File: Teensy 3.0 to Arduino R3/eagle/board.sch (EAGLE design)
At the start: 43 parts, among them IC1 7805TV, IC2 24AA256SN, IC3 24AA256SN, IC4 24AA256SN, IC5 24AA256SN, U1 MICROSD

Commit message: Version 3 final
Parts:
- added C9: (no value), resistor:CPOL-EUD
- added D2: (no value), SparkFun-DiscreteSemi:DIODESMA-KIT
- added R10, R11, R12, R13, R14, R15, R16, R17, R18, R19, R20, R21, R22, R23, R24, R5, R6, R7, R8, R9: (no value), resistor:R-EU_R0805
- added SJ3, SJ4, SJ5, SJ6: SOLDERJUMPERNO, SparkFun-Passives:SOLDERJUMPERNO
- IC1: value 7805TV -> 78XX compatible
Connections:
- removed net 3V3: C2.+, C4.1, C5.1, C6.1, C7.1, C8.1, IC1.VO, IC2.A2, IC2.VCC, IC3.A1, IC3.A2, IC3.VCC, IC4.A0, IC4.A2, IC4.VCC, IC5.A0, IC5.A1, IC5.A2, IC5.VCC, JP12.1, JP13.13, JP14.1, JP6.5, JP6.7, R1.2, R2.2, R3.2, R4.2, SJ2.1, U1.VDD
- new net N$10: JP2.7, R10.2
- new net N$11: JP2.6, R11.2
- new net N$12: JP2.5, R12.2
- new net N$13: JP1.13, R13.2
- new net N$14: JP1.12, R14.2
- new net N$15: JP1.11, R15.2
- new net N$16: JP1.10, R16.2
- new net N$17: JP1.9, R17.2
- new net N$18: JP1.8, R18.2
- new net N$19: JP1.7, R19.2
- new net N$20: JP1.6, R20.2
- new net N$21: JP2.4, R21.2
- new net N$22: JP2.3, R22.2
- new net N$23: JP2.2, R23.2
- new net N$24: JP2.1, R24.2
- new net N$5: JP1.5, R5.2
- new net N$6: JP1.4, R6.2
- new net N$7: JP1.3, R7.2
- new net N$8: JP1.2, R8.2
- new net N$9: JP1.1, R9.2
- new net NIC: R4.1, SJ3.1, SJ4.1, U1.CARD_DETECT
- new net QW: SJ5.1, SJ6.1, U1.CS
- net 3.3V: now also C2.+, C4.1, C5.1, C6.1, C7.1, C8.1, C9.+, D2.A, IC1.VO, IC2.A2, IC2.VCC, IC3.A1, IC3.A2, IC3.VCC, IC4.A0, IC4.A2, IC4.VCC, IC5.A0, IC5.A1, IC5.A2, IC5.VCC, JP12.1, JP13.13, JP14.1, JP6.5, JP6.7, R1.2, R2.2, R3.2, R4.2, SJ2.1, U1.VDD
- net A0: now also R23.1; no longer JP2.2
- net A1: now also R22.1; no longer JP2.3
- net A2: now also R21.1; no longer JP2.4
- net A3: now also R12.1; no longer JP2.5
- net A4: now also R11.1; no longer JP2.6
- net A5: now also R10.1; no longer JP2.7
- net D0: now also R13.1; no longer JP1.13
- net D1: now also R14.1; no longer JP1.12
- net D10: now also R7.1, SJ6.2; no longer JP1.3, U1.CS
- net D11: now also R8.1; no longer JP1.2
- net D12: now also R9.1; no longer JP1.1
- net D13: now also R24.1; no longer JP2.1
- net D2: now also R15.1; no longer JP1.11
- net D3: now also R16.1; no longer JP1.10
- net D4: now also R17.1; no longer JP1.9
- net D5: now also R18.1; no longer JP1.8
- net D6: now also R19.1; no longer JP1.7
- net D7: now also R20.1, SJ3.2; no longer JP1.6
- net D8: now also R5.1, SJ4.2; no longer JP1.5, R4.1, U1.CARD_DETECT
- net D9: now also R6.1, SJ5.2; no longer JP1.4
- net GND: now also C9.-
- net N$3: now also D2.C
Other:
- moved on the sheet: BAT1, C3, C4, F2, JP1, JP11, JP12, JP13, JP14, JP15, JP2, JP3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

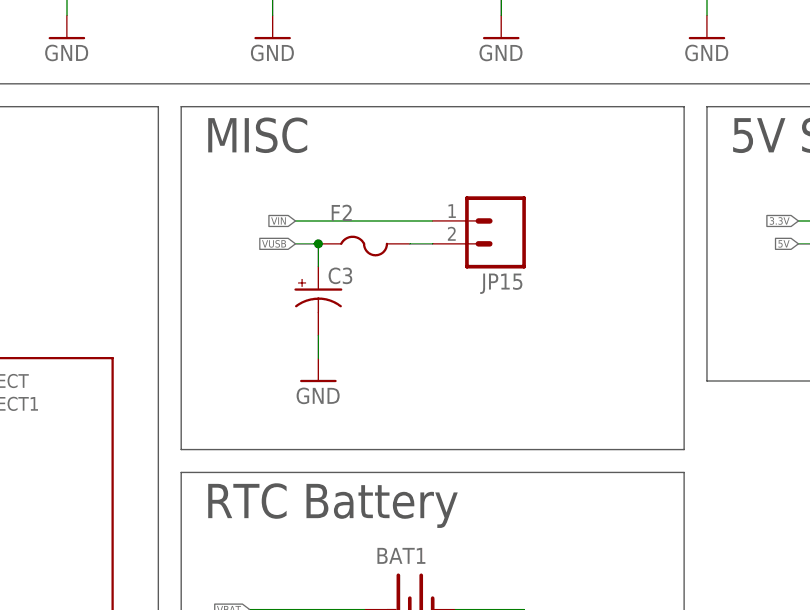
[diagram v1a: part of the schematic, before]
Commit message: V3-2: fixed several bugs
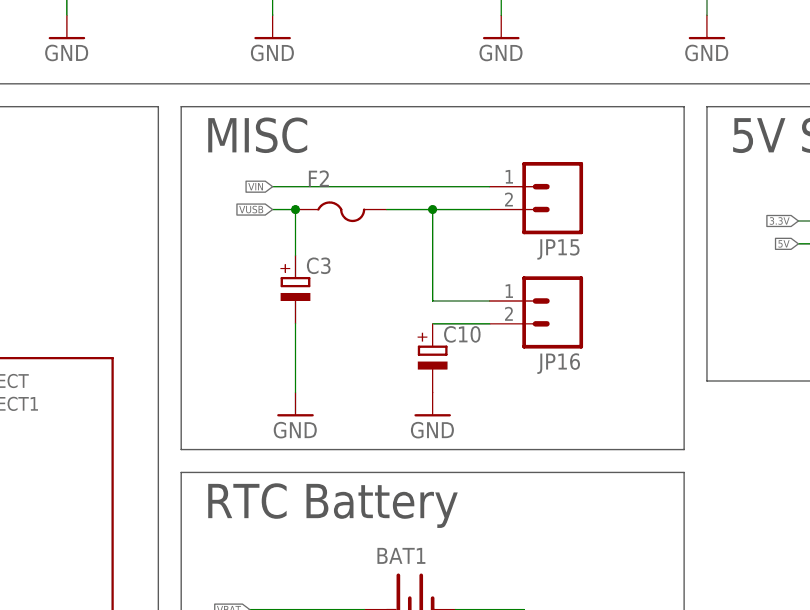
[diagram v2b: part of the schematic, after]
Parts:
- added C10: (no value), rcl:CPOL-EUSANYO_SMD_E7
- added JP16: (no value), SparkFun-Connectors:M02PTH
- C3: device SparkFun-Capacitors:CAP_POL3528-KIT -> rcl:CPOL-EUA/3216-18W
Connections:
- new net N$25: C10.+, JP16.2
- net GND: now also C10.-
- net N$2: now also JP16.1
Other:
- moved on the sheet: C3, F2, JP15
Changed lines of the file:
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@@
 <part name="F2" library="adafruit" deviceset="PTCFUSE" device="-1812"/>
 <part name="JP15" library="SparkFun-Connectors" deviceset="M02" device="PTH"/>
-<part name="C3" library="SparkFun-Capacitors" deviceset="CAP_POL" device="3528-KIT"/>
+<part name="C3" library="rcl" deviceset="CPOL-EU" device="A/3216-18W"/>
 <part name="GND1" library="SparkFun-Aesthetics" deviceset="GND" device=""/>
 <part name="GND2" library="SparkFun-Aesthetics" deviceset="GND" device=""/>
@@
 <part name="R23" library="resistor" deviceset="R-EU_" device="R0805"/>
 <part name="R24" library="resistor" deviceset="R-EU_" device="R0805"/>
+<part name="GND22" library="SparkFun-Aesthetics" deviceset="GND" device=""/>
+<part name="JP16" library="SparkFun-Connectors" deviceset="M02" device="PTH"/>
+<part name="C10" library="rcl" deviceset="CPOL-EU" device="SANYO_SMD_E7"/>
 </parts>
 <sheets>
@@
 <instance part="R3" gate="G$1" x="198.12" y="99.06" rot="R90"/>
 <instance part="P+3" gate="G$1" x="198.12" y="104.14"/>
-<instance part="F2" gate="G$1" x="393.7" y="99.06"/>
-<instance part="JP15" gate="G$1" x="408.94" y="104.14" rot="R180"/>
-<instance part="C3" gate="G$1" x="388.62" y="96.52"/>
-<instance part="GND1" gate="1" x="388.62" y="86.36"/>
+<instance part="F2" gate="G$1" x="391.16" y="102.87"/>
+<instance part="JP15" gate="G$1" x="415.29" y="107.95" rot="R180"/>
+<instance part="C3" gate="G$1" x="386.08" y="97.79"/>
+<instance part="GND1" gate="1" x="386.08" y="82.55"/>
 <instance part="GND2" gate="1" x="106.68" y="99.06"/>
 <instance part="GND3" gate="1" x="149.86" y="88.9"/>
@@
 <attribute name="VALUE" x="72.39" y="134.112" size="1.778" layer="96" rot="R180"/>
 </instance>
+<instance part="GND22" gate="1" x="401.32" y="82.55"/>
+<instance part="JP16" gate="G$1" x="415.29" y="95.25" rot="R180"/>
+<instance part="C10" gate="G$1" x="401.32" y="90.17"/>
 </instances>
 <busses>
@@
 <pinref part="C3" gate="G$1" pin="-"/>
 <pinref part="GND1" gate="1" pin="GND"/>
-<wire x1="388.62" y1="91.44" x2="388.62" y2="88.9" width="0.1524" layer="91"/>
+<wire x1="386.08" y1="92.71" x2="386.08" y2="85.09" width="0.1524" layer="91"/>
 </segment>
 <segment>
@@
 <wire x1="457.2" y1="147.32" x2="459.74" y2="147.32" width="0.1524" layer="91"/>
 </segment>
+<segment>
+<pinref part="GND22" gate="1" pin="GND"/>
+<pinref part="C10" gate="G$1" pin="-"/>
+</segment>
 </net>
 <net name="D0" class="0">
@@
 <segment>
 <pinref part="JP15" gate="G$1" pin="1"/>
-<wire x1="401.32" y1="104.14" x2="386.08" y2="104.14" width="0.1524" layer="91"/>
-<label x="386.08" y="104.14" size="0.8128" layer="95" rot="R180" xref="yes"/>
+<wire x1="407.67" y1="107.95" x2="383.54" y2="107.95" width="0.1524" layer="91"/>
+<label x="383.54" y="107.95" size="0.8128" layer="95" rot="R180" xref="yes"/>
 </segment>
 </net>
@@
 <segment>
 <pinref part="F2" gate="G$1" pin="1"/>
-<wire x1="388.62" y1="101.6" x2="386.08" y2="101.6" width="0.1524" layer="91"/>
-<label x="386.08" y="101.6" size="0.8128" layer="95" rot="R180" xref="yes"/>
+<wire x1="386.08" y1="105.41" x2="383.54" y2="105.41" width="0.1524" layer="91"/>
+<label x="383.54" y="105.41" size="0.8128" layer="95" rot="R180" xref="yes"/>
 <pinref part="C3" gate="G$1" pin="+"/>
-<wire x1="388.62" y1="99.06" x2="388.62" y2="101.6" width="0.1524" layer="91"/>
-<junction x="388.62" y="101.6"/>
+<wire x1="386.08" y1="100.33" x2="386.08" y2="105.41" width="0.1524" layer="91"/>
+<junction x="386.08" y="105.41"/>
 </segment>
 </net>
@@
 <pinref part="F2" gate="G$1" pin="2"/>
 <pinref part="JP15" gate="G$1" pin="2"/>
-<wire x1="398.78" y1="101.6" x2="401.32" y2="101.6" width="0.1524" layer="91"/>
+<wire x1="396.24" y1="105.41" x2="401.32" y2="105.41" width="0.1524" layer="91"/>
+<pinref part="JP16" gate="G$1" pin="1"/>
+<wire x1="401.32" y1="105.41" x2="407.67" y2="105.41" width="0.1524" layer="91"/>
+<wire x1="407.67" y1="95.25" x2="401.32" y2="95.25" width="0.1524" layer="91"/>
+<wire x1="401.32" y1="95.25" x2="401.32" y2="105.41" width="0.1524" layer="91"/>
+<junction x="401.32" y="105.41"/>
 </segment>
 </net>
@@
 </segment>
 </net>
+<net name="N$25" class="0">
+<segment>
+<pinref part="C10" gate="G$1" pin="+"/>
+<pinref part="JP16" gate="G$1" pin="2"/>
+<wire x1="401.32" y1="92.71" x2="407.67" y2="92.71" width="0.1524" layer="91"/>
+</segment>
+</net>
